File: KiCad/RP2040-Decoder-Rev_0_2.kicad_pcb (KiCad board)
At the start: 2 copper layers, 25 x 20 mm, 44 parts, among them J1 DCC_IN, J2 MOTOR_CONN, J3 GPIO_CONN, J4 DEBUG_CONN, Q1 WNM2030, Q2 WNM2030, Q3 WNM2030, Q4 WNM2030, U1 PJ75AL33SA, U2 BDR6133, U3 W25Q64JVSSIQ, U4 RP2040, Y1 X322512MSB4SI

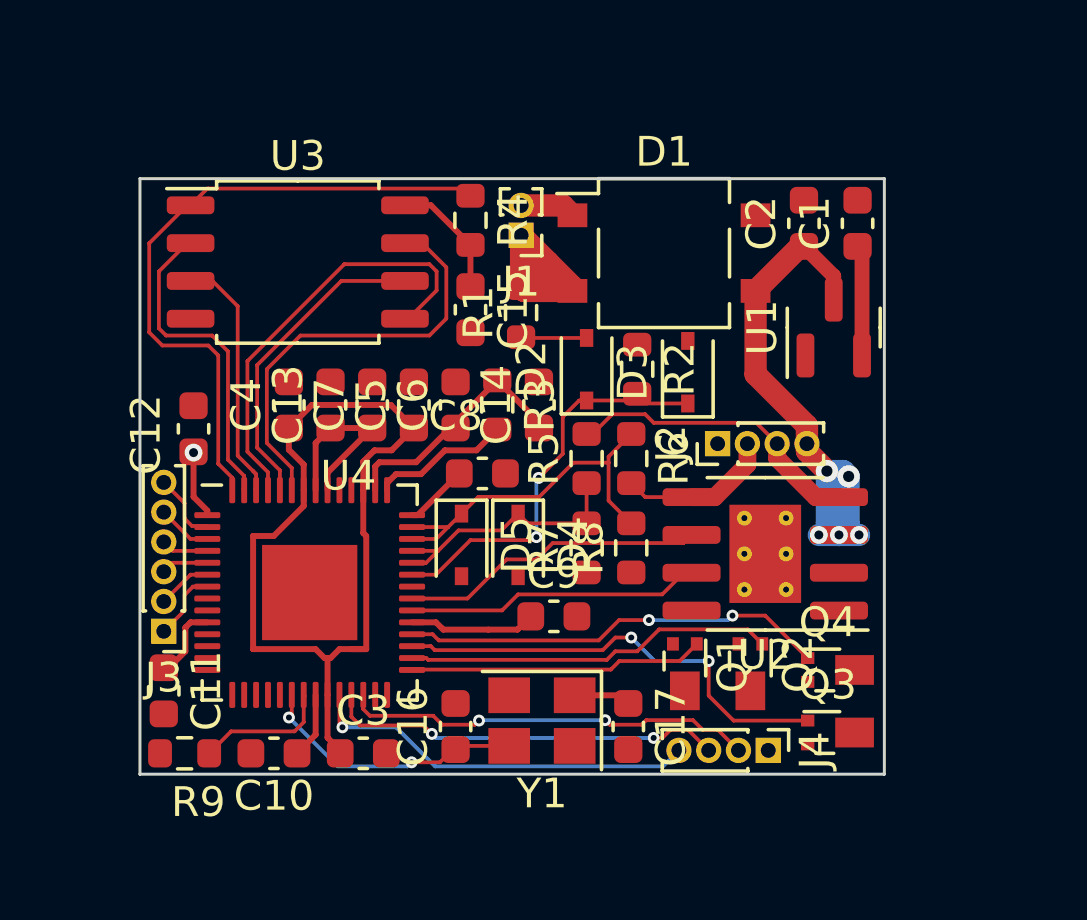
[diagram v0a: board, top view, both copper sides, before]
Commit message: Finished Board
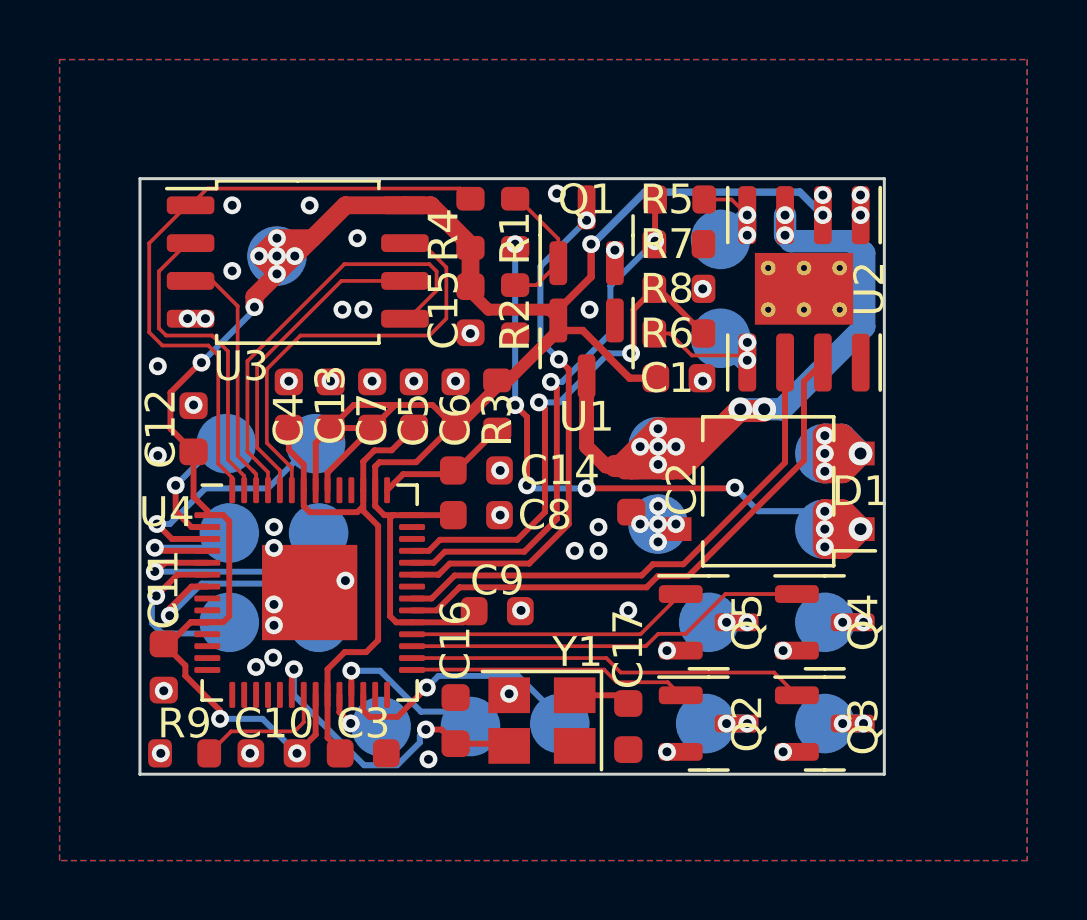
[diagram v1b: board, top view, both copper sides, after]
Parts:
- removed D2: 1N4148WS, Diode_SMD:D_SOD-323
- removed D3, D4, D5: BZT52C3V3S, Diode_SMD:D_SOD-323
- added J10: 2, TestPoint:TestPoint_Pad_D2.0mm, B.Cu at (140.5, 101.9)
- added J11: 3, TestPoint:TestPoint_Pad_D2.0mm, B.Cu at (143.5, 101.9)
- added J12: 4, TestPoint:TestPoint_Pad_D2.0mm, B.Cu at (140.5, 104.9)
- added J13: 5, TestPoint:TestPoint_Pad_D2.0mm, B.Cu at (143.5, 104.9)
- added J14: +V, TestPoint:TestPoint_Pad_D2.0mm, B.Cu at (154.9, 99.0)
- added J15: M_OUT_B, TestPoint:TestPoint_Pad_D2.0mm, B.Cu at (157.0, 92.0)
- added J16: M_OUT_A, TestPoint:TestPoint_Pad_D2.0mm, B.Cu at (157.0, 95.4)
- added J17: GND, TestPoint:TestPoint_Pad_D2.0mm, B.Cu at (154.9, 101.6)
- added J18: SWCLK, TestPoint:TestPoint_Pad_D2.0mm, B.Cu at (145.6, 108.4)
- added J19: SWDIO, TestPoint:TestPoint_Pad_D2.0mm, B.Cu at (148.6, 108.4)
- added J20: RUN, TestPoint:TestPoint_Pad_D2.0mm, B.Cu at (151.6, 108.3)
- added J5: 2, TestPoint:TestPoint_Pad_D2.0mm, B.Cu at (160.5, 104.9)
- added J6: 3, TestPoint:TestPoint_Pad_D2.0mm, B.Cu at (156.6, 104.9)
- added J7: +3V3, TestPoint:TestPoint_Pad_D2.0mm, B.Cu at (142.1, 92.6)
- added J8: 0, TestPoint:TestPoint_Pad_D2.0mm, B.Cu at (140.4, 98.9)
- added J9: 1, TestPoint:TestPoint_Pad_D2.0mm, B.Cu at (143.4, 98.9)
- added Q5: T2N7002BK, Package_TO_SOT_SMD:SOT-23, F.Cu at (156.6, 104.9)
- C1, C10, C11, C12, C13, C15, C16, C17, C2, C3, C4, C7, C8, C9: footprint Capacitor_SMD:C_0603_1608Metric -> RP2040-Decoder_Additional_Footprints:C_0603_1608Metric
- C14, C5, C6: value 2u2 -> 10u; footprint Capacitor_SMD:C_0603_1608Metric -> RP2040-Decoder_Additional_Footprints:C_0603_1608Metric
- J1: value DCC_IN -> T0; footprint Connector_PinHeader_1.00mm:PinHeader_1x02_P1.00mm_Vertical -> TestPoint:TestPoint_Pad_D2.0mm; moved to B.Cu
- J2: value MOTOR_CONN -> T1; footprint Connector_PinHeader_1.00mm:PinHeader_1x04_P1.00mm_Vertical -> TestPoint:TestPoint_Pad_D2.0mm; moved to B.Cu
- J3: value GPIO_CONN -> 0; footprint Connector_PinHeader_1.00mm:PinHeader_1x06_P1.00mm_Vertical -> TestPoint:TestPoint_Pad_D2.0mm; moved to B.Cu
- J4: value DEBUG_CONN -> 1; footprint Connector_PinHeader_1.00mm:PinHeader_1x04_P1.00mm_Vertical -> TestPoint:TestPoint_Pad_D2.0mm; moved to B.Cu
- Q1, Q2, Q3, Q4: value WNM2030 -> T2N7002BK; footprint RP2040-Decoder_Additional_Footprints:SOT-723-Extended_Pad -> Package_TO_SOT_SMD:SOT-23
- R1, R5, R6: value 10k -> 6k8; footprint Resistor_SMD:R_0603_1608Metric -> RP2040-Decoder_Additional_Footprints:R_0603_1608Metric
- R2: value 47k -> 6k8; footprint Resistor_SMD:R_0603_1608Metric -> RP2040-Decoder_Additional_Footprints:R_0603_1608Metric
- R3, R4, R9: footprint Resistor_SMD:R_0603_1608Metric -> RP2040-Decoder_Additional_Footprints:R_0603_1608Metric
- R7, R8: value 10k -> 1k; footprint Resistor_SMD:R_0603_1608Metric -> RP2040-Decoder_Additional_Footprints:R_0603_1608Metric
- U2: footprint Package_SO:SOIC-8-1EP_3.9x4.9mm_P1.27mm_EP2.41x3.3mm_ThermalVias -> RP2040-Decoder_Additional_Footprints:SOIC-8-1EP_3.9x4.9mm_P1.27mm_EP2.41x3.3mm_ThermalVias
- U3: footprint Package_SO:SOIC-8_5.23x5.23mm_P1.27mm -> RP2040-Decoder_Additional_Footprints:SOIC-8_5.23x5.23mm_P1.27mm
- moved J3 18.5 mm to (156.5, 108.3)
- moved Q1 14.7 mm to (152.5, 91.9), turned to 90 degrees
- moved J1 14.2 mm to (160.5, 101.8)
- moved R7 10.7 mm to (155.6, 92.2), turned to 180 degrees
- moved C2 10.6 mm to (154.0, 100.4), turned to -90 degrees
- moved R5 9.24 mm to (155.6, 90.7), turned to 0 degrees
- moved U2 8.99 mm to (159.8, 93.7), turned to -90 degrees
- moved R8 8.85 mm to (155.6, 93.7), turned to 180 degrees
- moved D1 8.73 mm to (158.6, 100.5), turned to 180 degrees
- moved U1 8.33 mm to (152.5, 95.7), turned to -90 degrees
- moved C1 7.94 mm to (155.6, 96.7), turned to 0 degrees
- moved R2 4.56 mm to (150.1, 94.4), turned to 90 degrees
- moved R6 4.49 mm to (155.6, 95.2), turned to 180 degrees
- moved J2 3.62 mm to (160.5, 99.2), turned to 180 degrees
- moved C14 3.04 mm to (148.8, 99.8), turned to 0 degrees
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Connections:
- C2 pad 1: +12V -> +V
- D1 pad 3: +12V -> +V
- J1 pad 1: Net-(D1-Pad2) -> Net-(D1-Pad1)
- J2 pad 1: GND -> Net-(D1-Pad2)
- J4 pad 1: GND -> Net-(J4-Pad1)
- Q1 pad 1: /GPIO18 -> Net-(Q1-Pad1)
- Q1 pad 3: unconnected-(Q1-Pad3) -> /GPIO24
- Q2 pad 1: /GPIO19 -> /GPIO18
- Q2 pad 3: unconnected-(Q2-Pad3) -> Net-(J3-Pad1)
- Q3 pad 1: /GPIO20 -> /GPIO19
- Q3 pad 3: unconnected-(Q3-Pad3) -> Net-(J4-Pad1)
- Q4 pad 1: /GPIO21 -> /GPIO20
- Q4 pad 3: unconnected-(Q4-Pad3) -> Net-(J5-Pad1)
- R1 pad 1: Net-(D2-Pad2) -> Net-(Q1-Pad1)
- R1 pad 2: Net-(D1-Pad2) -> Net-(D1-Pad1)
- R2 pad 2: /GPIO24 -> Net-(Q1-Pad1)
- U1 pad 3: +12V -> +V
- U2 pad 3: +12V -> +V
- U4 pad 2: Net-(J3-Pad6) -> Net-(J8-Pad1)
- U4 pad 24: Net-(J4-Pad4) -> Net-(J18-Pad1)
- U4 pad 25: Net-(J4-Pad3) -> Net-(J19-Pad1)
- U4 pad 26: Net-(J4-Pad2) -> Net-(J20-Pad1)
- U4 pad 3: Net-(J3-Pad5) -> Net-(J9-Pad1)
- U4 pad 39: /ADC_EMF_A -> /ADC_EMF_B
- U4 pad 4: Net-(J3-Pad4) -> Net-(J10-Pad1)
- U4 pad 40: /ADC_EMF_B -> unconnected-(U4-Pad40)
- U4 pad 41: /ADC_EMF_B -> unconnected-(U4-Pad41)
- U4 pad 5: Net-(J3-Pad3) -> Net-(J11-Pad1)
- U4 pad 6: Net-(J3-Pad2) -> Net-(J12-Pad1)
- U4 pad 7: Net-(J3-Pad1) -> Net-(J13-Pad1)
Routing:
- net +3V3: track 36.0 -> 93.2 mm, vias 1 -> 12
- net +V: track 0.00 -> 34.5 mm, vias 0 -> 9
- net Net-(D1-Pad1): track 1.86 -> 28.5 mm, vias 0 -> 9
- net +12V: track 18.1 -> 0.00 mm, vias 5 -> 0
- net Net-(J4-Pad2): track 13.9 -> 0.00 mm, vias 2 -> 0
- net Net-(J4-Pad3): track 13.4 -> 0.00 mm, vias 2 -> 0
- net Net-(J4-Pad4): track 13.2 -> 0.00 mm, vias 1 -> 0
- net +1V1: track 29.9 -> 18.4 mm
- net /ADC_EMF_A: track 8.90 -> 18.1 mm, vias 0 -> 2
- net /GPIO22: track 9.91 -> 18.8 mm
- net Net-(J20-Pad1): track 0.00 -> 8.57 mm, vias 0 -> 1
- net Net-(J9-Pad1): track 0.00 -> 8.30 mm, vias 0 -> 1
- net Net-(J11-Pad1): track 0.00 -> 7.88 mm, vias 0 -> 1
- net Net-(J13-Pad1): track 0.00 -> 7.82 mm, vias 0 -> 1
- net /GPIO23: track 10.3 -> 17.8 mm
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- added copper zone on B.Cu, net GND
- added copper zone on F.Cu, net GND
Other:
- board text added: "AUX"
- board text added: "DEBUG"
- board text added: "GPIO"
- board text added: "Gabriel Koppenstein RP2040-Decoder"
- board text added: "M"
- board text added: "Rev. 0.2"
